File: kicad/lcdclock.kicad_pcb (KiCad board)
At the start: 2 copper layers, 41 x 50 mm, 28 parts, among them J1 Conn_JLink_SWD, Q1 BSH205, SW1 SW_Push, U1 STM32L073xx_48, U2 ELV_DCF-2, U3 TPS70630, U4 LCD, Y1 32.768kHz 12.5pF

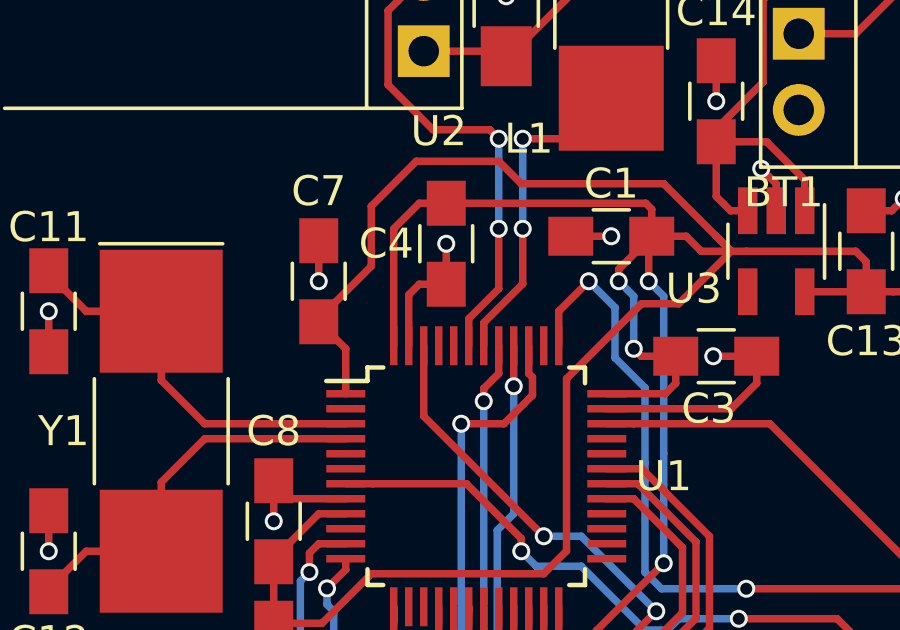
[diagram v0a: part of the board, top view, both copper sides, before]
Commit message: Final fixes
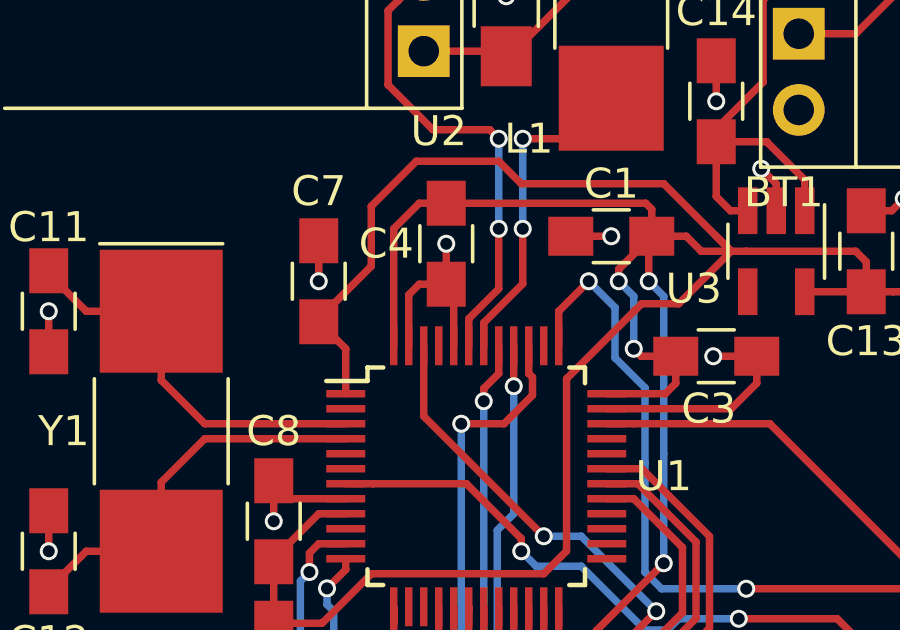
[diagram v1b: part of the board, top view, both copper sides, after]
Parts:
- BT1: value 4xAA 6.4-3.2V -> 4xAAA 6.4-3.2V
- R1: value 100k -> ?
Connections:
- J1 pad 11: (no net) -> Net-(J1-Pad11)
- J1 pad 13: (no net) -> Net-(J1-Pad13)
- J1 pad 17: (no net) -> Net-(J1-Pad17)
- J1 pad 19: (no net) -> Net-(J1-Pad19)
- J1 pad 2: (no net) -> Net-(J1-Pad2)
- J1 pad 3: (no net) -> Net-(J1-Pad3)
- J1 pad 5: (no net) -> Net-(J1-Pad5)
- U1 pad 25: (no net) -> Net-(U1-Pad25)
- U1 pad 26: (no net) -> Net-(U1-Pad26)
- U1 pad 27: (no net) -> Net-(U1-Pad27)
- U1 pad 28: (no net) -> Net-(U1-Pad28)
- U1 pad 38: (no net) -> Net-(U1-Pad38)
- U1 pad 44: (no net) -> GND
- U1 pad 45: (no net) -> Net-(U1-Pad45)
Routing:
- net GND: track 45.9 -> 48.1 mm
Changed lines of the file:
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@@
 (kicad_pcb (version 4) (host pcbnew 4.0.7)
   (general
-    (links 83)
+    (links 84)
     (no_connects 0)
     (area 19.924999 19.924999 61.075001 70.075001)
     (thickness 1.6)
     (drawings 5)
-    (tracks 375)
+    (tracks 377)
     (zones 0)
     (modules 28)
-    (nets 32)
+    (nets 45)
   )
   (page A4)
@@
   (net 30 "Net-(C14-Pad1)")
   (net 31 "Net-(Q1-Pad1)")
+  (net 32 "Net-(J1-Pad2)")
+  (net 33 "Net-(J1-Pad3)")
+  (net 34 "Net-(J1-Pad5)")
+  (net 35 "Net-(J1-Pad11)")
+  (net 36 "Net-(J1-Pad13)")
+  (net 37 "Net-(J1-Pad17)")
+  (net 38 "Net-(J1-Pad19)")
+  (net 39 "Net-(U1-Pad25)")
+  (net 40 "Net-(U1-Pad26)")
+  (net 41 "Net-(U1-Pad27)")
+  (net 42 "Net-(U1-Pad28)")
+  (net 43 "Net-(U1-Pad38)")
+  (net 44 "Net-(U1-Pad45)")
   (net_class Default "This is the default net class."
     (clearance 0.2)
@@
     (add_net "Net-(C5-Pad2)")
     (add_net "Net-(D1-Pad2)")
+    (add_net "Net-(J1-Pad11)")
+    (add_net "Net-(J1-Pad13)")
+    (add_net "Net-(J1-Pad17)")
+    (add_net "Net-(J1-Pad19)")
+    (add_net "Net-(J1-Pad2)")
+    (add_net "Net-(J1-Pad3)")
+    (add_net "Net-(J1-Pad5)")
     (add_net "Net-(J1-Pad7)")
     (add_net "Net-(J1-Pad9)")
@@
     (add_net "Net-(U1-Pad21)")
     (add_net "Net-(U1-Pad22)")
+    (add_net "Net-(U1-Pad25)")
+    (add_net "Net-(U1-Pad26)")
+    (add_net "Net-(U1-Pad27)")
+    (add_net "Net-(U1-Pad28)")
     (add_net "Net-(U1-Pad29)")
     (add_net "Net-(U1-Pad30)")
     (add_net "Net-(U1-Pad31)")
+    (add_net "Net-(U1-Pad38)")
     (add_net "Net-(U1-Pad39)")
     (add_net "Net-(U1-Pad40)")
     (add_net "Net-(U1-Pad41)")
     (add_net "Net-(U1-Pad43)")
+    (add_net "Net-(U1-Pad45)")
     (add_net "Net-(U1-Pad46)")
     (add_net VCC)
@@
     (pad 1 thru_hole rect (at 0 0 90) (size 1.7272 1.7272) (drill 1.016) (layers *.Cu *.Mask)
       (net 5 VCC))
-    (pad 2 thru_hole oval (at 0 -2.54 90) (size 1.7272 1.7272) (drill 1.016) (layers *.Cu *.Mask))
-    (pad 3 thru_hole oval (at 2.54 0 90) (size 1.7272 1.7272) (drill 1.016) (layers *.Cu *.Mask))
+    (pad 2 thru_hole oval (at 0 -2.54 90) (size 1.7272 1.7272) (drill 1.016) (layers *.Cu *.Mask)
+      (net 32 "Net-(J1-Pad2)"))
+    (pad 3 thru_hole oval (at 2.54 0 90) (size 1.7272 1.7272) (drill 1.016) (layers *.Cu *.Mask)
+      (net 33 "Net-(J1-Pad3)"))
     (pad 4 thru_hole oval (at 2.54 -2.54 90) (size 1.7272 1.7272) (drill 1.016) (layers *.Cu *.Mask)
       (net 2 GND))
-    (pad 5 thru_hole oval (at 5.08 0 90) (size 1.7272 1.7272) (drill 1.016) (layers *.Cu *.Mask))
+    (pad 5 thru_hole oval (at 5.08 0 90) (size 1.7272 1.7272) (drill 1.016) (layers *.Cu *.Mask)
+      (net 34 "Net-(J1-Pad5)"))
     (pad 6 thru_hole oval (at 5.08 -2.54 90) (size 1.7272 1.7272) (drill 1.016) (layers *.Cu *.Mask)
       (net 2 GND))
@@
     (pad 10 thru_hole oval (at 10.16 -2.54 90) (size 1.7272 1.7272) (drill 1.016) (layers *.Cu *.Mask)
       (net 2 GND))
-    (pad 11 thru_hole oval (at 12.7 0 90) (size 1.7272 1.7272) (drill 1.016) (layers *.Cu *.Mask))
+    (pad 11 thru_hole oval (at 12.7 0 90) (size 1.7272 1.7272) (drill 1.016) (layers *.Cu *.Mask)
+      (net 35 "Net-(J1-Pad11)"))
     (pad 12 thru_hole oval (at 12.7 -2.54 90) (size 1.7272 1.7272) (drill 1.016) (layers *.Cu *.Mask)
       (net 2 GND))
-    (pad 13 thru_hole oval (at 15.24 0 90) (size 1.7272 1.7272) (drill 1.016) (layers *.Cu *.Mask))
+    (pad 13 thru_hole oval (at 15.24 0 90) (size 1.7272 1.7272) (drill 1.016) (layers *.Cu *.Mask)
+      (net 36 "Net-(J1-Pad13)"))
     (pad 14 thru_hole oval (at 15.24 -2.54 90) (size 1.7272 1.7272) (drill 1.016) (layers *.Cu *.Mask)
       (net 2 GND))
@@
     (pad 16 thru_hole oval (at 17.78 -2.54 90) (size 1.7272 1.7272) (drill 1.016) (layers *.Cu *.Mask)
       (net 2 GND))
-    (pad 17 thru_hole oval (at 20.32 0 90) (size 1.7272 1.7272) (drill 1.016) (layers *.Cu *.Mask))
+    (pad 17 thru_hole oval (at 20.32 0 90) (size 1.7272 1.7272) (drill 1.016) (layers *.Cu *.Mask)
+      (net 37 "Net-(J1-Pad17)"))
     (pad 18 thru_hole oval (at 20.32 -2.54 90) (size 1.7272 1.7272) (drill 1.016) (layers *.Cu *.Mask)
       (net 2 GND))
-    (pad 19 thru_hole oval (at 22.86 0 90) (size 1.7272 1.7272) (drill 1.016) (layers *.Cu *.Mask))
+    (pad 19 thru_hole oval (at 22.86 0 90) (size 1.7272 1.7272) (drill 1.016) (layers *.Cu *.Mask)
+      (net 38 "Net-(J1-Pad19)"))
     (pad 20 thru_hole oval (at 22.86 -2.54 90) (size 1.7272 1.7272) (drill 1.016) (layers *.Cu *.Mask)
       (net 2 GND))
@@
       (effects (font (size 1 1) (thickness 0.15)))
     )
-    (fp_text value 100k (at 0 1.75 90) (layer F.Fab)
+    (fp_text value ? (at 0 1.75 90) (layer F.Fab)
       (effects (font (size 1 1) (thickness 0.15)))
     )
@@
     (pad 24 smd rect (at 2.75 4.35 90) (size 1.3 0.25) (layers F.Cu F.Paste F.Mask)
       (net 5 VCC))
-    (pad 25 smd rect (at 4.35 2.75) (size 1.3 0.25) (layers F.Cu F.Paste F.Mask))
-    (pad 26 smd rect (at 4.35 2.25) (size 1.3 0.25) (layers F.Cu F.Paste F.Mask))
-    (pad 27 smd rect (at 4.35 1.75) (size 1.3 0.25) (layers F.Cu F.Paste F.Mask))
-    (pad 28 smd rect (at 4.35 1.25) (size 1.3 0.25) (layers F.Cu F.Paste F.Mask))
+    (pad 25 smd rect (at 4.35 2.75) (size 1.3 0.25) (layers F.Cu F.Paste F.Mask)
+      (net 39 "Net-(U1-Pad25)"))
+    (pad 26 smd rect (at 4.35 2.25) (size 1.3 0.25) (layers F.Cu F.Paste F.Mask)
+      (net 40 "Net-(U1-Pad26)"))
+    (pad 27 smd rect (at 4.35 1.75) (size 1.3 0.25) (layers F.Cu F.Paste F.Mask)
+      (net 41 "Net-(U1-Pad27)"))
+    (pad 28 smd rect (at 4.35 1.25) (size 1.3 0.25) (layers F.Cu F.Paste F.Mask)
+      (net 42 "Net-(U1-Pad28)"))
     (pad 29 smd rect (at 4.35 0.75) (size 1.3 0.25) (layers F.Cu F.Paste F.Mask)
       (net 22 "Net-(U1-Pad29)"))
@@
     (pad 37 smd rect (at 2.75 -4.35 90) (size 1.3 0.25) (layers F.Cu F.Paste F.Mask)
       (net 11 "Net-(J1-Pad9)"))
-    (pad 38 smd rect (at 2.25 -4.35 90) (size 1.3 0.25) (layers F.Cu F.Paste F.Mask))
+    (pad 38 smd rect (at 2.25 -4.35 90) (size 1.3 0.25) (layers F.Cu F.Paste F.Mask)
+      (net 43 "Net-(U1-Pad38)"))
     (pad 39 smd rect (at 1.75 -4.35 90) (size 1.3 0.25) (layers F.Cu F.Paste F.Mask)
       (net 25 "Net-(U1-Pad39)"))
@@
     (pad 43 smd rect (at -0.25 -4.35 90) (size 1.3 0.25) (layers F.Cu F.Paste F.Mask)
       (net 29 "Net-(U1-Pad43)"))
-    (pad 44 smd rect (at -0.75 -4.35 90) (size 1.3 0.25) (layers F.Cu F.Paste F.Mask))
-    (pad 45 smd rect (at -1.25 -4.35 90) (size 1.3 0.25) (layers F.Cu F.Paste F.Mask))
+    (pad 44 smd rect (at -0.75 -4.35 90) (size 1.3 0.25) (layers F.Cu F.Paste F.Mask)
+      (net 2 GND))
+    (pad 45 smd rect (at -1.25 -4.35 90) (size 1.3 0.25) (layers F.Cu F.Paste F.Mask)
+      (net 44 "Net-(U1-Pad45)"))
     (pad 46 smd rect (at -1.75 -4.35 90) (size 1.3 0.25) (layers F.Cu F.Paste F.Mask)
       (net 28 "Net-(U1-Pad46)"))
@@
       (effects (font (size 1 1) (thickness 0.15)))
     )
-    (fp_text value "4xAA 6.4-3.2V" (at 1.905 -4.445 270) (layer F.Fab)
+    (fp_text value "4xAAA 6.4-3.2V" (at 1.905 -4.445 270) (layer F.Fab)
       (effects (font (size 1 1) (thickness 0.15)))
     )
@@
   (segment (start 52.25 23.15) (end 52.25 22.5) (width 0.25) (layer F.Cu) (net 1))
   (segment (start 46.75 27.5) (end 46.75 26.75) (width 0.25) (layer F.Cu) (net 1))
+  (segment (start 35.25 37.15) (end 35.25 35.35) (width 0.25) (layer F.Cu) (net 2))
+  (segment (start 35.25 35.35) (end 35 35.1) (width 0.25) (layer F.Cu) (net 2))
   (segment (start 43.9 21.75) (end 45.25 21.75) (width 0.25) (layer F.Cu) (net 2))
   (via (at 45.25 21.75) (size 0.6) (drill 0.4) (layers F.Cu B.Cu) (net 2))
